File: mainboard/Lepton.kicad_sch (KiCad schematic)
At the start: 15 parts, among them IC1001 TXB0104RUT, IC1002 PCA9306JK, IC1003 TXB0104RUT, X1001 LEPTON, Y1001 25 MHz

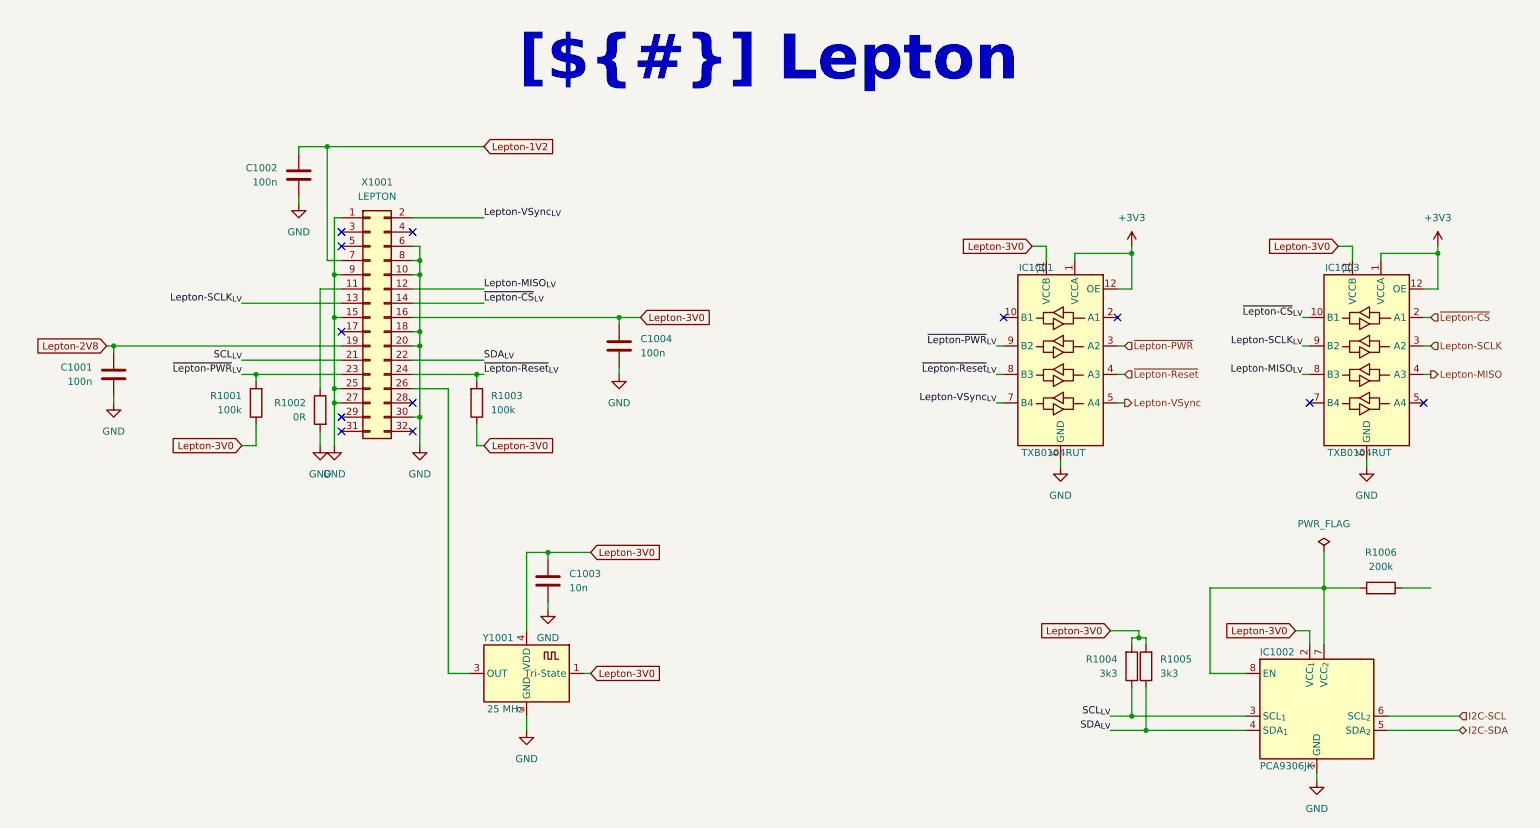
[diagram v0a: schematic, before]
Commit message: Layout complete
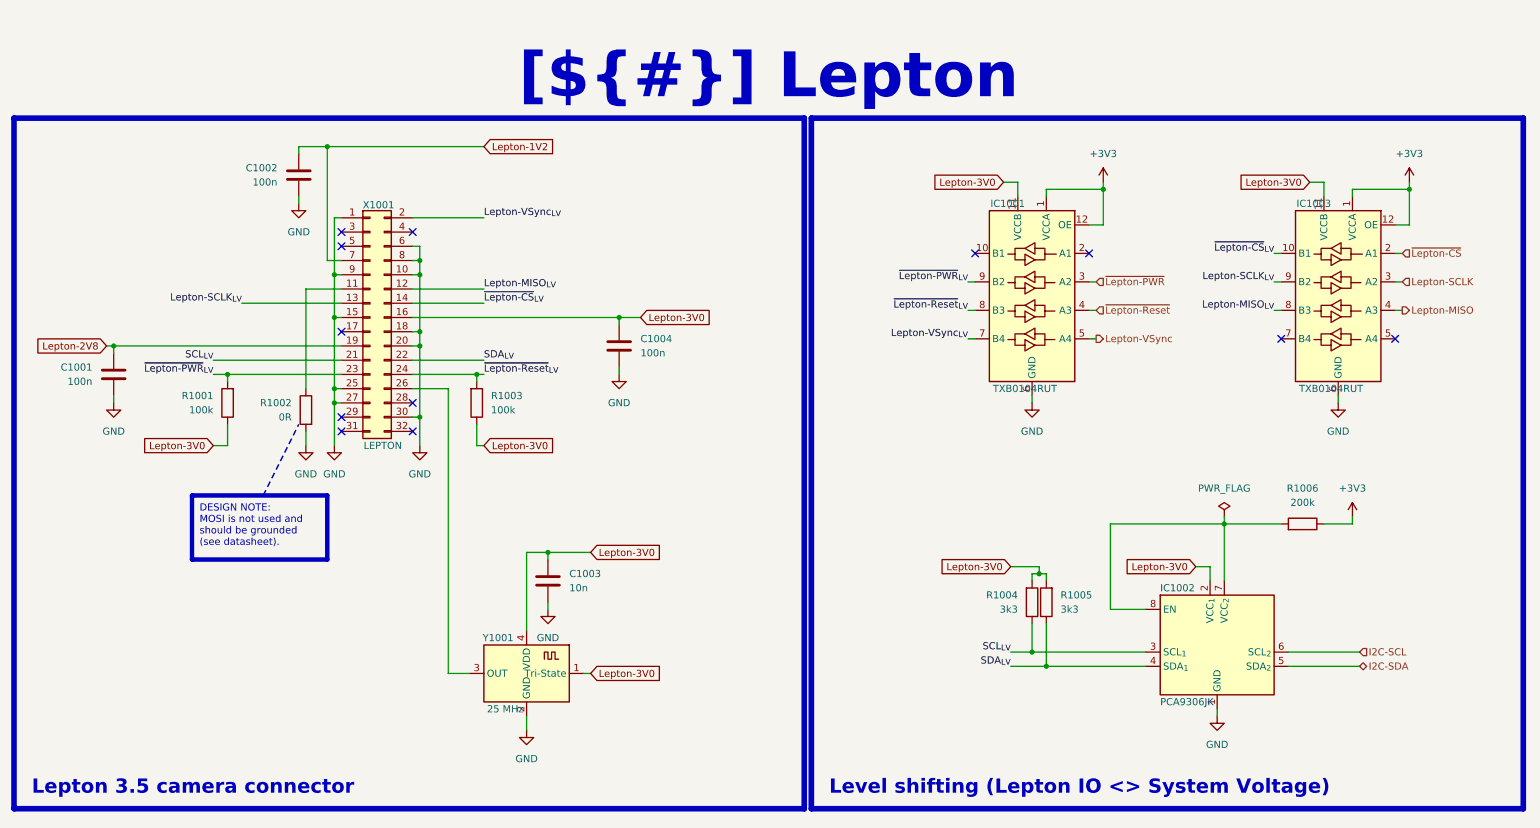
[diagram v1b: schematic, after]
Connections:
- net +3V3: now also R1006.1
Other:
- moved on the sheet: IC1001, IC1002, IC1003, R1001, R1002, R1004, R1005, R1006
